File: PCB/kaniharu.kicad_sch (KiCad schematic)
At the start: 13 parts, among them J1 RJ45_Bel_SI-60062-F, U1 STM32H743ZITx, U3 DP83822IRHBR, Y2 Crystal_GND24_Small

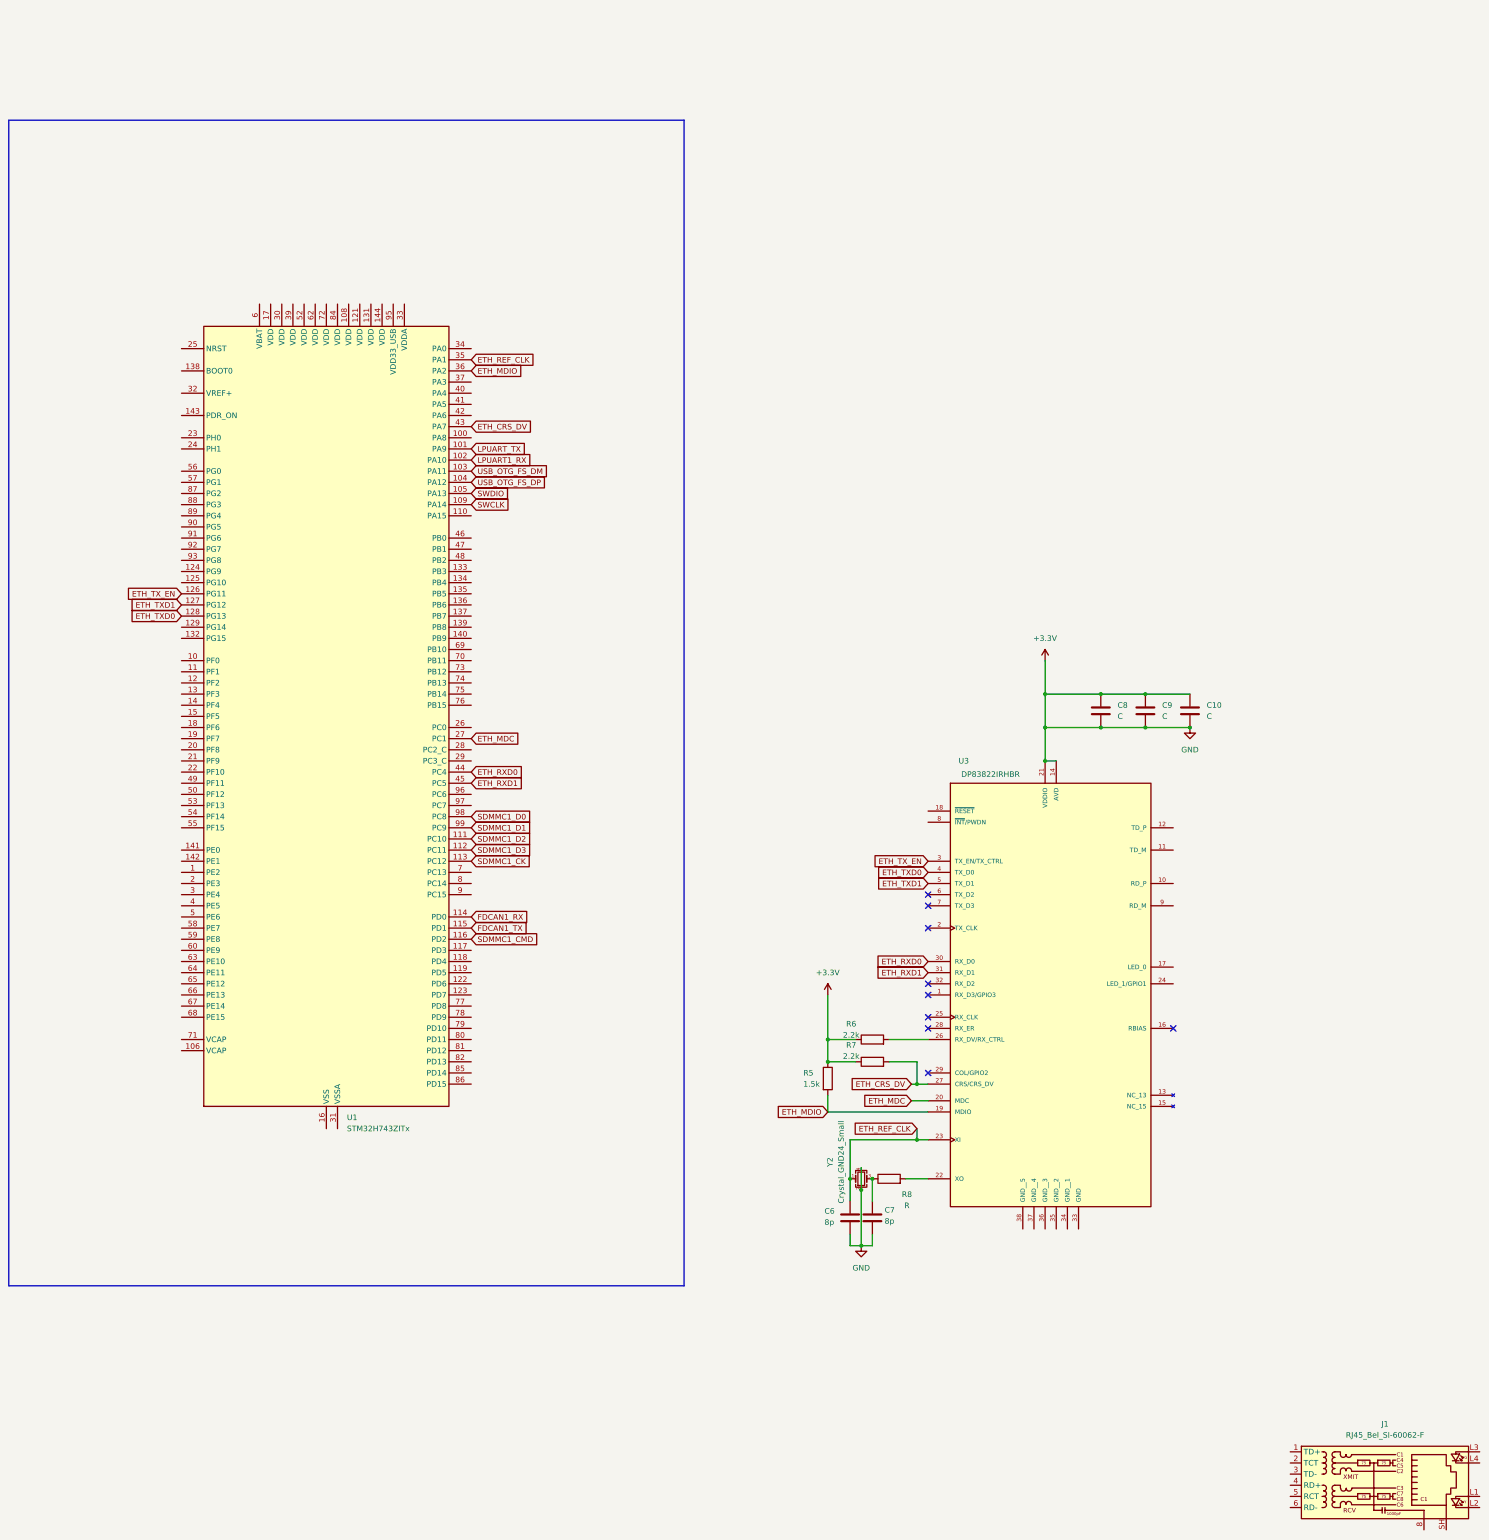
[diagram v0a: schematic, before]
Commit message: update
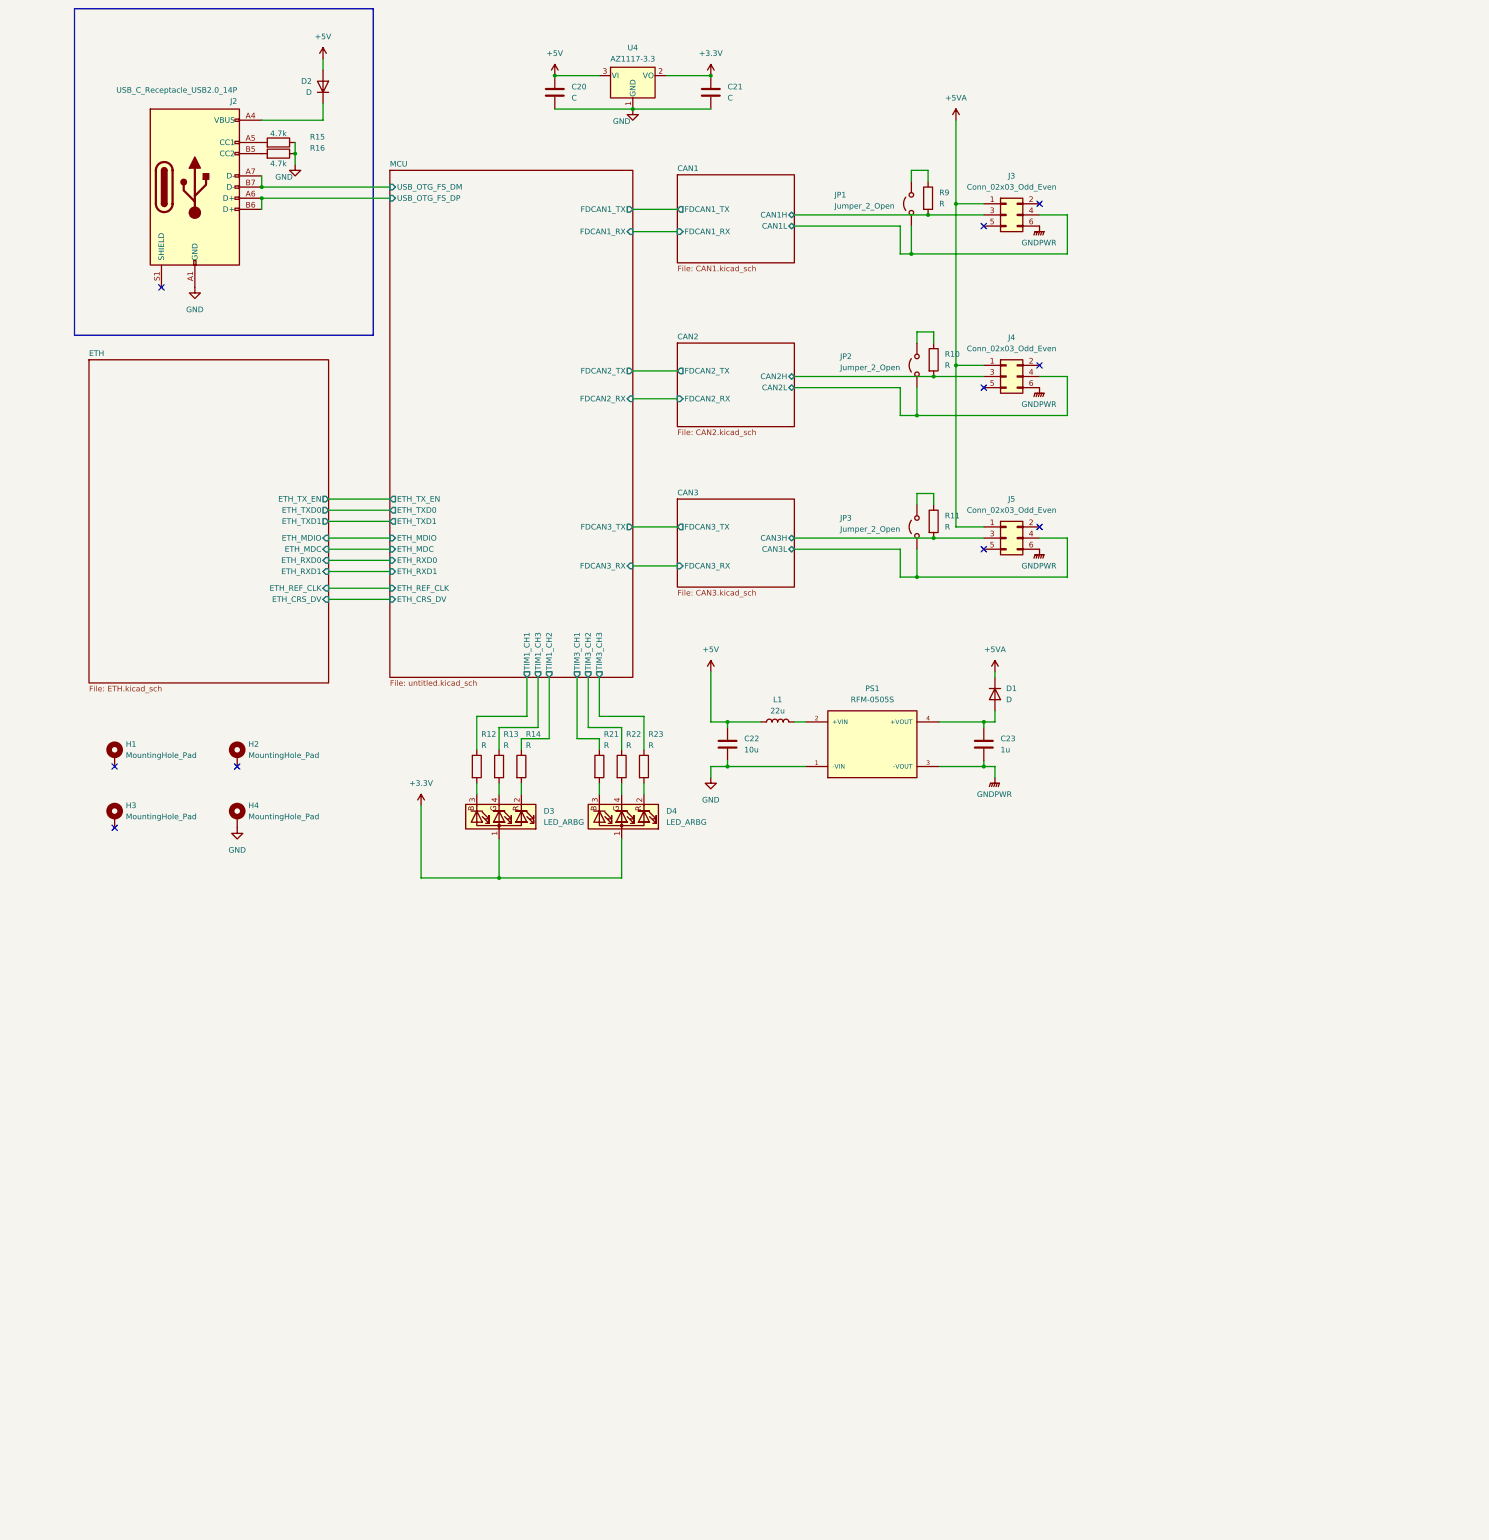
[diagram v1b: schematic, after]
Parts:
- removed C10, C8, C9: C, symbol Device:C
- removed C6, C7: 8p, symbol Device:C
- removed J1: RJ45_Bel_SI-60062-F, Connector_RJ:RJ45_Bel_SI-60062-F, symbol Connector:RJ45_Bel_SI-60062-F
- removed R5: 1.5k, symbol Device:R
- removed R6, R7: 2.2k, symbol Device:R
- removed R8: R, symbol Device:R
- removed U1: STM32H743ZITx, Package_QFP:LQFP-144_20x20mm_P0.5mm, symbol MCU_ST_STM32H7:STM32H743ZITx
- removed U3: DP83822IRHBR, DP83822IRHBR:IC_DP83822IRHBR, symbol 0_mylib:DP83822IRHBR
- removed Y2: Crystal_GND24_Small, symbol Device:Crystal_GND24_Small
- added C20, C21: C, Capacitor_SMD:C_0805_2012Metric_Pad1.18x1.45mm_HandSolder, symbol Device:C
- added C22: 10u, Capacitor_SMD:C_0805_2012Metric_Pad1.18x1.45mm_HandSolder, symbol Device:C
- added C23: 1u, Capacitor_SMD:C_0603_1608Metric_Pad1.08x0.95mm_HandSolder, symbol Device:C
- added D1, D2: D, 0_syslib:SODFL3618X110N, symbol Device:D
- added D3, D4: LED_ARBG, 0_syslib:OSTB0603C1CA, symbol Device:LED_ARBG
- added H1, H2, H3: MountingHole_Pad, MountingHole:MountingHole_3.2mm_M3, symbol Mechanical:MountingHole_Pad
- added H4: MountingHole_Pad, MountingHole:MountingHole_3.2mm_M3_Pad, symbol Mechanical:MountingHole_Pad
- added J2: USB_C_Receptacle_USB2.0_14P, Connector_USB:USB_C_Receptacle_HRO_TYPE-C-31-M-12, symbol Connector:USB_C_Receptacle_USB2.0_14P
- added J3, J4, J5: Conn_02x03_Odd_Even, Connector_IDC:IDC-Header_2x03_P2.54mm_Horizontal, symbol Connector_Generic:Conn_02x03_Odd_Even
- added JP1, JP2, JP3: Jumper_2_Open, Connector_PinHeader_2.54mm:PinHeader_1x02_P2.54mm_Vertical, symbol Jumper:Jumper_2_Open
- added L1: 22u, Inductor_SMD:L_0805_2012Metric_Pad1.15x1.40mm_HandSolder, symbol Device:L
- added PS1: RFM-0505S, 0_mylib:RFM-0505S, symbol 0_mylib:RFM-0505S
- added R10, R11, R12, R13, R14, R21, R22, R23, R9: R, Resistor_SMD:R_0402_1005Metric_Pad0.72x0.64mm_HandSolder, symbol Device:R
- added R15: 4.7k, Resistor_SMD:R_0603_1608Metric, symbol Device:R
- added R16: 4.7k, Resistor_SMD:R_0402_1005Metric_Pad0.72x0.64mm_HandSolder, symbol Device:R
- added U4: AZ1117-3.3, Package_TO_SOT_SMD:SOT-223-3_TabPin2, symbol Regulator_Linear:AZ1117-3.3
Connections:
- net +3.3V: now also C21.1, D3.1 (A), D4.1 (A), U4.2 (VO)
- new net: JP1.2 (B), R9.1
- new net: JP2.2 (B), R10.1
- new net: D4.2 (RK), R23.2
- new net: D4.3 (BK), R21.2
- new net: D4.4 (GK), R22.2
- new net: C23.1, D1.2 (A), PS1.4 (+VOUT)
- new net: D3.2 (RK), R14.2
- new net: D3.3 (BK), R12.2
- new net: D3.4 (GK), R13.2
- new net: D2.1 (K), J2.A4 (VBUS), J2.A9 (VBUS), J2.B4 (VBUS), J2.B9 (VBUS)
- new net: J2.A5 (CC1), R15.2
- new net: J2.B5 (CC2), R16.2
- new net: L1.2, PS1.2 (+VIN)
- new net: JP3.2 (B), R11.1
- new net +5V: C20.1, C22.1, D2.2 (A), L1.1, U4.3 (VI)
- new net +5VA: D1.1 (K), J3.1 (Pin_1), J4.1 (Pin_1), J5.1 (Pin_1)
- new net CAN1/CAN1H: J3.3 (Pin_3), R9.2
- new net CAN1/CAN1L: J3.4 (Pin_4), JP1.1 (A)
- new net CAN2/CAN2H: J4.3 (Pin_3), R10.2
- new net CAN2/CAN2L: J4.4 (Pin_4), JP2.1 (A)
- new net CAN3/CAN3H: J5.3 (Pin_3), R11.2
- new net CAN3/CAN3L: J5.4 (Pin_4), JP3.1 (A)
- new net GND: C20.2, C21.2, C22.2, H4.1, J2.A1 (GND), J2.A12 (GND), J2.B1 (GND), J2.B12 (GND), PS1.1 (-VIN), R15.1, R16.1, U4.1 (GND)
- new net GNDPWR: C23.2, J3.6 (Pin_6), J4.6 (Pin_6), J5.6 (Pin_6), PS1.3 (-VOUT)
- new net MCU/TIM1_CH1: R12.1
- new net MCU/TIM1_CH2: R14.1
- new net MCU/TIM1_CH3: R13.1
- new net MCU/TIM3_CH1: R21.1
- new net MCU/TIM3_CH2: R22.1
- new net MCU/TIM3_CH3: R23.1
- new net MCU/USB_OTG_FS_DM: J2.A7 (D-), J2.B7 (D-)
- new net MCU/USB_OTG_FS_DP: J2.A6 (D+), J2.B6 (D+)
- no-connect marks 9 -> 10
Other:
- added sheet CAN1 (CAN1.kicad_sch)
- added sheet CAN2 (CAN2.kicad_sch)
- added sheet CAN3 (CAN3.kicad_sch)
- added sheet ETH (ETH.kicad_sch)
- added sheet MCU (untitled.kicad_sch)
